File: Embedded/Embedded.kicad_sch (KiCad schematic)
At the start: 59 parts, among them J1 GyroBreakout, J10 TouchButton, J11 USB-C Breakout, J2 BaseResMUX, J3 BaseNeoMUX, J4 HelixNeo, J5 FanConnector, J6 Conn_01x08, J7 Conn_01x08, J8 Speaker, J9 LightSensor, Q1 FQP27P06, SW1 BackboardSw, SW2 BackboardSw, U1 ESP32-C6-WROOM-1, U2 BQ25895RTW, U3 FSUSB30MUX, U5 MP8715, U7 SN74AHCT125N, U8 SN74AHCT125N

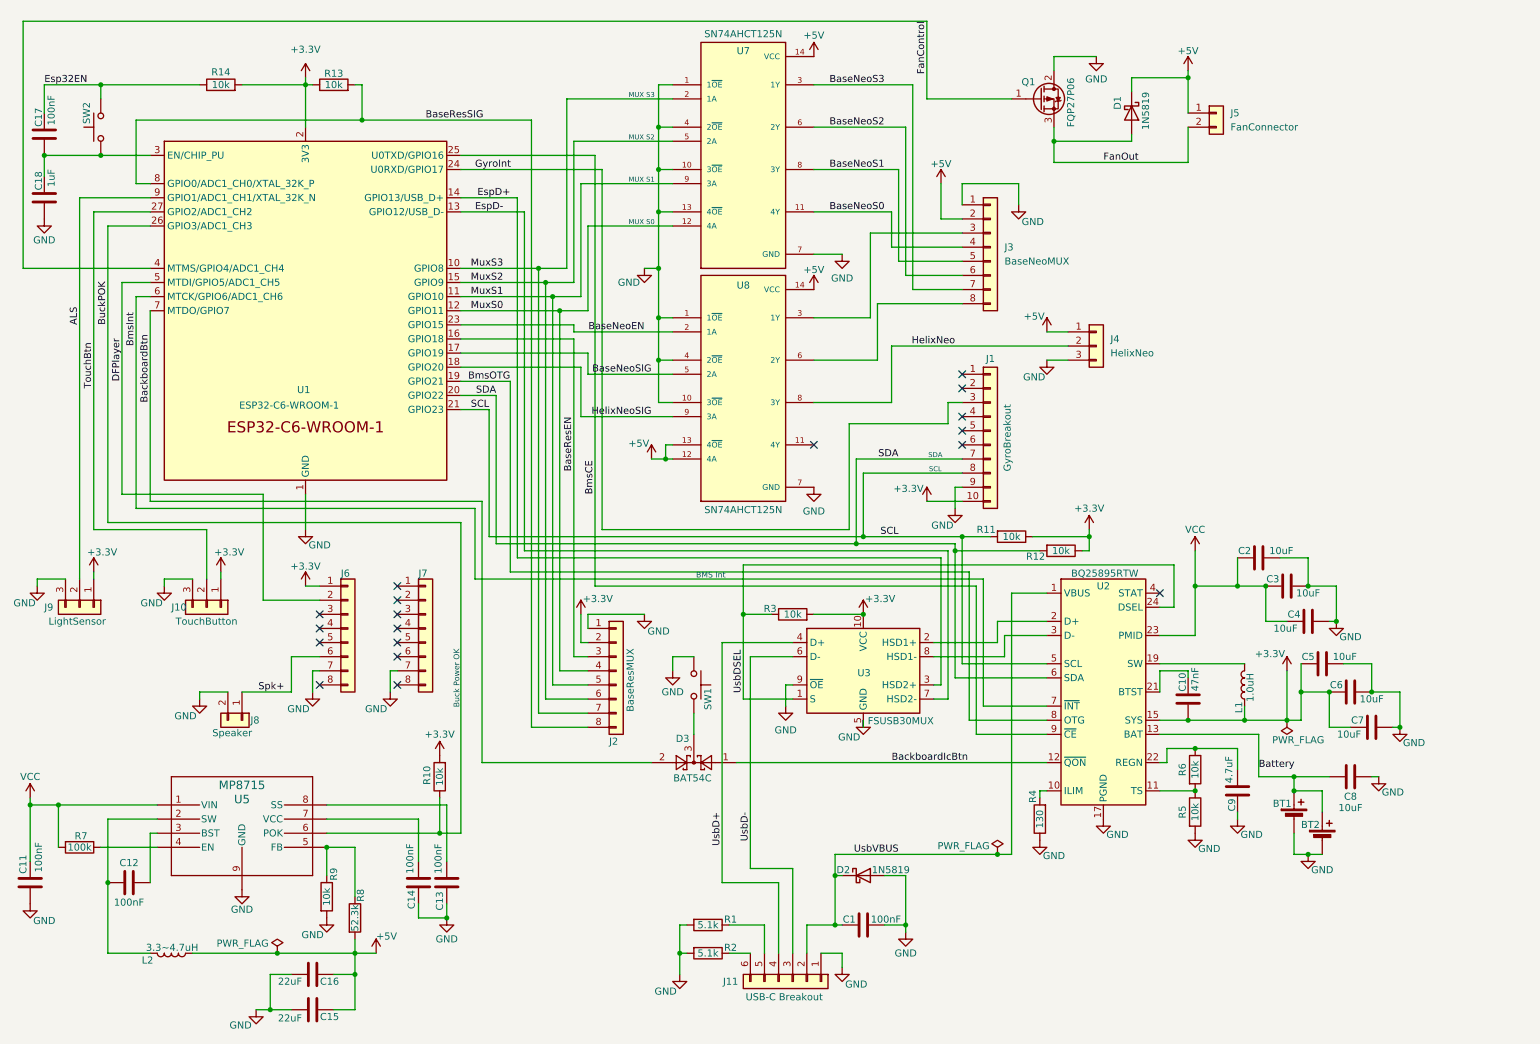
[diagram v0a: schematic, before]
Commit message: v4
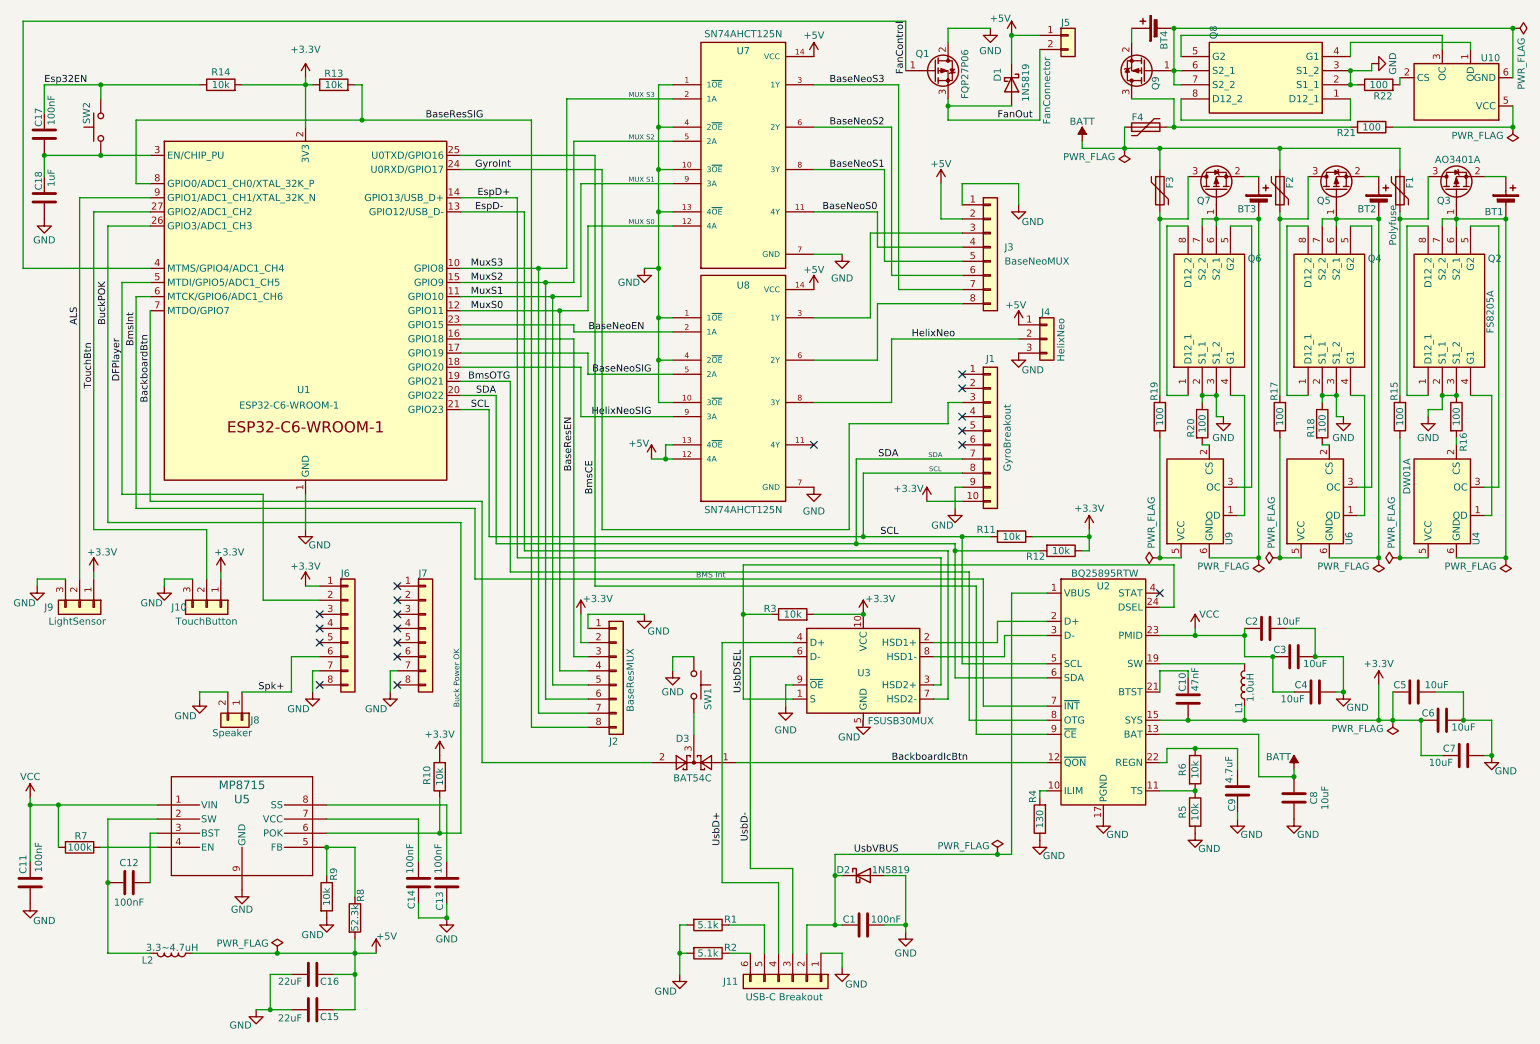
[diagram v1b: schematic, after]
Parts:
- added BT3, BT4: Battery_Cell, Connector_JST:JST_PH_B2B-PH-K_1x02_P2.00mm_Vertical, symbol Device:Battery_Cell
- added F1, F2, F3, F4: Polyfuse, Fuse:Fuse_1206_3216Metric_Pad1.42x1.75mm_HandSolder, symbol Device:Polyfuse
- added Q2, Q4, Q6, Q8: FS8205A, Package_SO:MSOP-8_3x3mm_P0.65mm, symbol symbols:FS8205A
- added Q3, Q5, Q7, Q9: AO3401A, Package_TO_SOT_SMD:TSOT-23_HandSoldering, symbol Transistor_FET:AO3401A
- added R15, R16, R17, R18, R19, R20, R21, R22: 100, Resistor_THT:R_Axial_DIN0207_L6.3mm_D2.5mm_P10.16mm_Horizontal, symbol Device:R
- added U10, U4, U6, U9: DW01A, Package_TO_SOT_SMD:SOT-23-6, symbol Battery_Management:DW01A
- BT1, BT2: footprint Capacitor_SMD:C_1808_4520Metric_Pad1.72x2.30mm_HandSolder -> Connector_JST:JST_PH_B2B-PH-K_1x02_P2.00mm_Vertical
- Q1: footprint Package_TO_SOT_THT:TO-220-3_Vertical -> Package_TO_SOT_THT:TO-220-3_Horizontal_TabDown
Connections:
- net GND: now also C8.1, Q2.2 (S1_1), Q2.3 (S1_2), Q4.2 (S1_1), Q4.3 (S1_2), Q6.2 (S1_1), Q6.3 (S1_2), Q8.2 (S1_1), Q8.3 (S1_2), R16.1, R18.1, R20.1, R22.1; no longer BT1.2 (-), BT2.2 (-), C8.2
- removed net Battery: BT1.1 (+), BT2.1 (+), C8.1, U2.13 (BAT), U2.14 (BAT)
- new net: R18.2, U6.2 (CS)
- new net: Q6.1 (D12_1), Q6.8 (D12_2)
- new net: Q6.4 (G1), U9.1 (OD)
- new net: Q6.5 (G2), U9.3 (OC)
- new net: BT3.2 (-), Q6.6 (S2_1), Q6.7 (S2_2), Q7.1 (G), U9.6 (GND)
- new net: R20.2, U9.2 (CS)
- new net: R19.1, U9.5 (VCC)
- new net: BT2.1 (+), Q5.2 (S)
- new net: BT2.2 (-), Q4.6 (S2_1), Q4.7 (S2_2), Q5.1 (G), U6.6 (GND)
- new net: Q4.1 (D12_1), Q4.8 (D12_2)
- new net: Q4.4 (G1), U6.1 (OD)
- new net: Q4.5 (G2), U6.3 (OC)
- new net: R16.2, U4.2 (CS)
- new net: BT4.2 (-), Q8.6 (S2_1), Q8.7 (S2_2), Q9.1 (G), U10.6 (GND)
- new net: BT4.1 (+), Q9.2 (S)
- new net: F4.2, Q9.3 (D), R21.2
- new net: Q8.4 (G1), U10.1 (OD)
- new net: R22.2, U10.2 (CS)
- new net: Q8.5 (G2), U10.3 (OC)
- new net: R21.1, U10.5 (VCC)
- new net: R17.1, U6.5 (VCC)
- new net: F2.2, Q5.3 (D), R17.2
- new net: Q2.4 (G1), U4.1 (OD)
- new net: Q2.5 (G2), U4.3 (OC)
- new net: R15.1, U4.5 (VCC)
- new net: BT1.2 (-), Q2.6 (S2_1), Q2.7 (S2_2), Q3.1 (G), U4.6 (GND)
- new net: F1.2, Q3.3 (D), R15.2
- new net: BT1.1 (+), Q3.2 (S)
- new net: F3.2, Q7.3 (D), R19.2
- new net: BT3.1 (+), Q7.2 (S)
- new net: Q2.1 (D12_1), Q2.8 (D12_2)
- new net: Q8.1 (D12_1), Q8.8 (D12_2)
- new net BATT: C8.2, F1.1, F2.1, F3.1, F4.1, U2.13 (BAT), U2.14 (BAT)
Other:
- moved on the sheet: C2, C3, C4, C5, C6, C7, C8, D1, J4, J5, Q1
